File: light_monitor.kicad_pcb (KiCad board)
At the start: 2 copper layers, 32.9 x 32.9 mm, 15 parts, among them IC1 TSL25911FN, U1 STM32L432KCUx, U2 STDC14, U5 RV-8803-C7, X1 board_lens

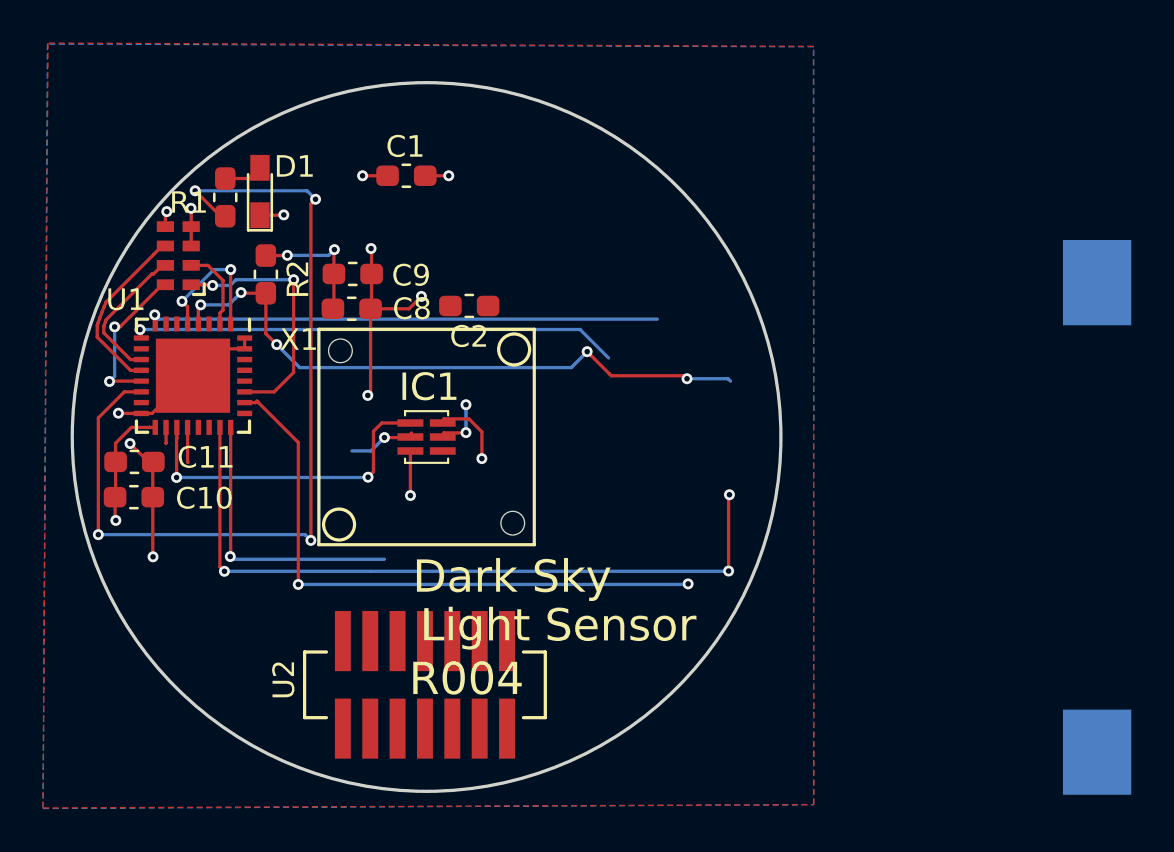
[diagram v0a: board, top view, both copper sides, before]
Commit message: r004 board added
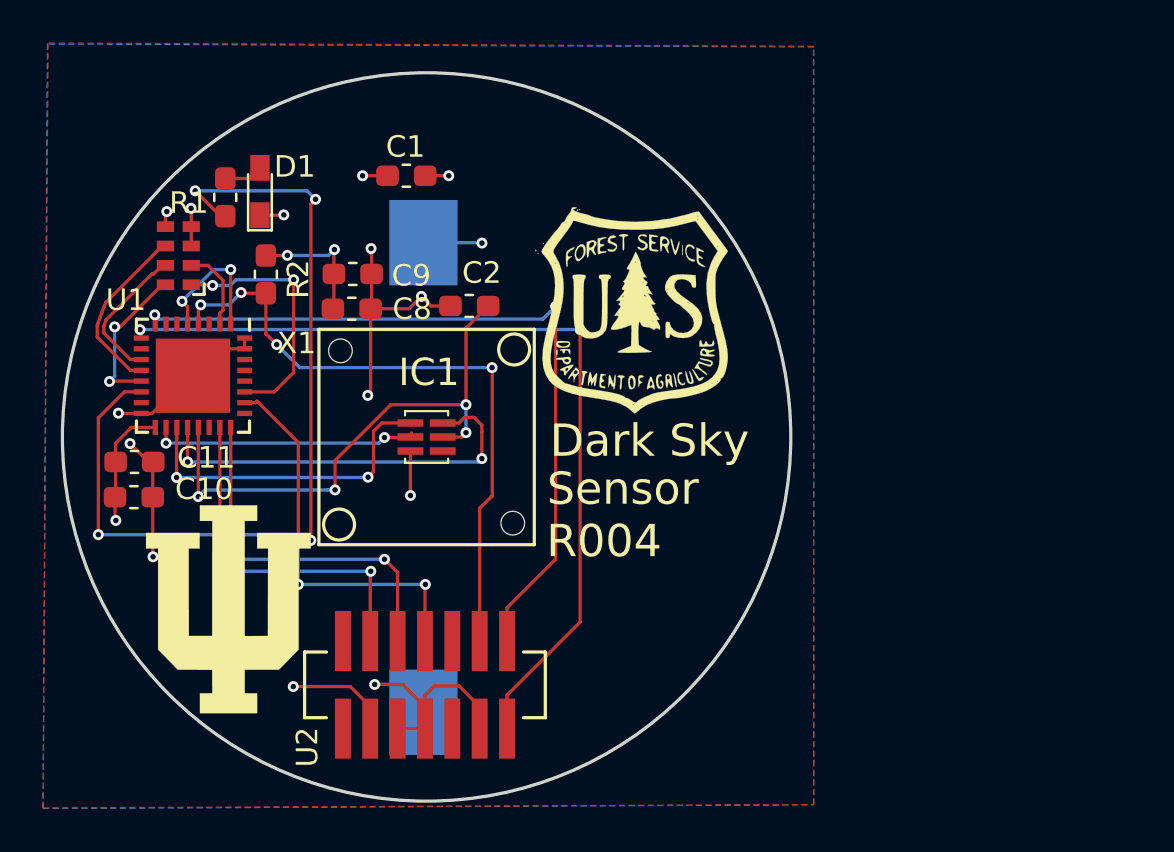
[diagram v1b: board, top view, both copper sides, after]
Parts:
- added G***: LOGO, logo:iu_trident, F.Cu at (104.2, 113.2)
- added G***: LOGO, logo:hnf_logo, F.Cu at (123.0, 99.4)
- moved BT1 31.3 mm to (113.2, 107.1)
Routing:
- net /sensor_power: track 2.54 -> 25.8 mm, vias 2 -> 4
- net /RX: track 22.7 -> 40.8 mm, vias 1 -> 2
- net /SWDIO: track 33.7 -> 16.8 mm, vias 3 -> 2
- net GND: track 30.8 -> 45.8 mm, vias 10 -> 11
- net /sensor_data: track 5.10 -> 19.0 mm, vias 1 -> 2
- net /TX: track 23.8 -> 35.8 mm, vias 1 -> 2
- net /SWO: track 28.0 -> 18.6 mm
- net /sensor_int: track 3.72 -> 12.2 mm, vias 1 -> 2
- net VDD: track 21.3 -> 29.0 mm, vias 7 -> 9
- net /SWDCLK: track 13.2 -> 17.3 mm, vias 1 -> 2
- net /NRST: track 29.2 -> 30.2 mm, vias 5 -> 4
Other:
- board size 32.9 x 32.9 mm -> 33.8 x 33.8 mm
- board text added: "Sensor"
- board text removed: "Light Sensor"
